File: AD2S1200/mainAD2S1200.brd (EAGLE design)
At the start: 100 x 80 mm, 36 parts, among them IC1 OPA1013D, IC2 OPA1013D, Q1(9235.11QRTZ) 8.192, X1 22-23-2041

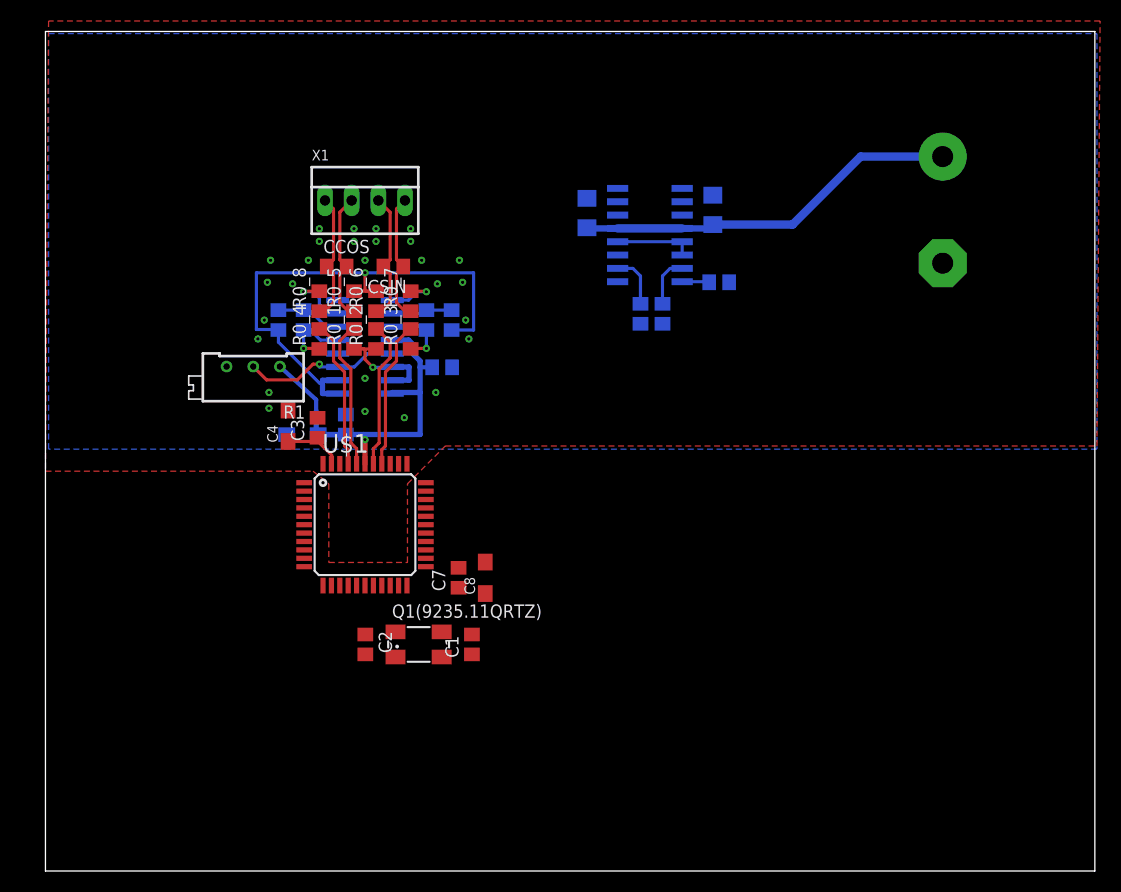
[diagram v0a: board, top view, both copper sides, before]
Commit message: Ok
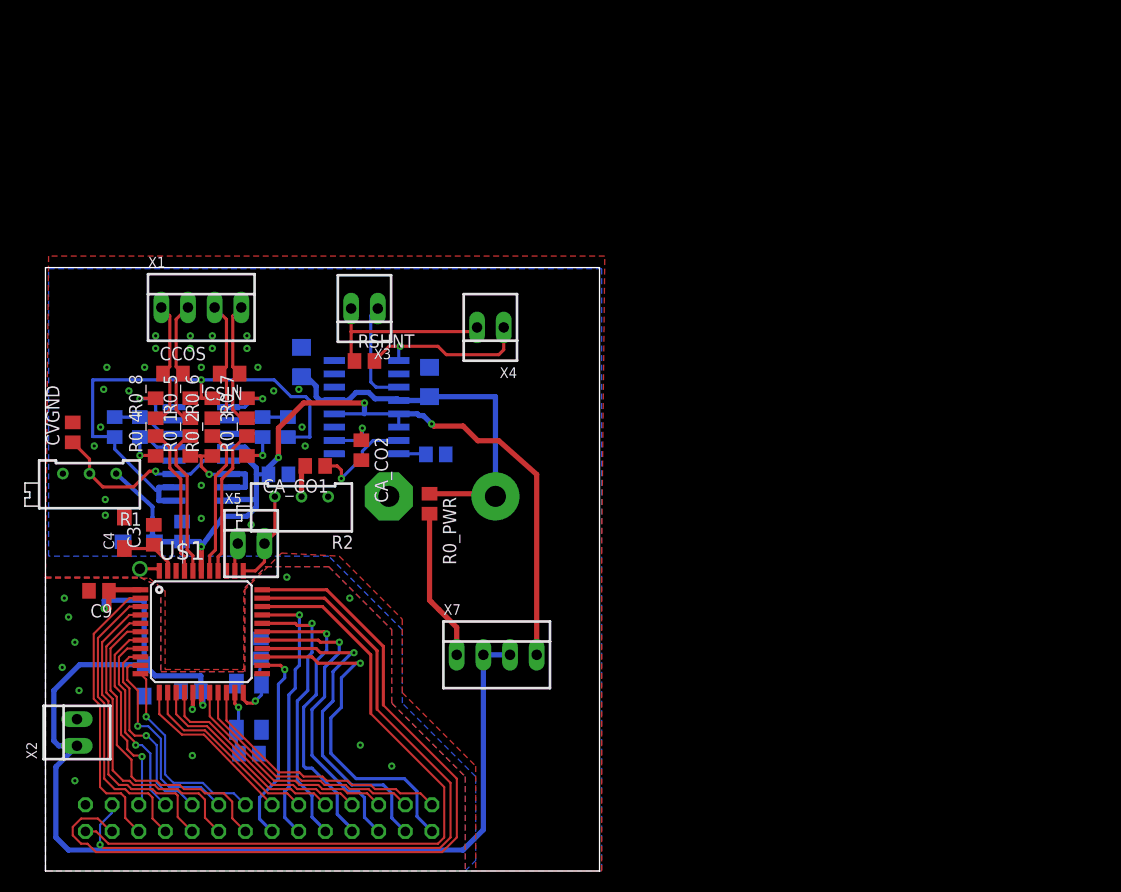
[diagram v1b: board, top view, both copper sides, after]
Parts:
- added C9: 100n, rcl:C0805
- added CVGND: (no value), rcl:C0805
- added R0_PWR, RSHNT: (no value), resistor:R0805
- added R2: (no value), resistor:RTRIM64X
- added SV3, SV4: (no value), con-ml:ML14
- added X2, X3, X4, X5: 22-23-2021, con-molex:22-23-2021
- added X7: 22-23-2041, con-molex:22-23-2041
- moved CA1 55.0 mm to (37.8, 35.7), turned to 0 degrees
- moved CA_CO1 36.1 mm to (25.7, 38.6), flipped to the top, turned to 180 degrees
- moved C8 33.9 mm to (9.41, 18.2), flipped to the bottom, turned to 270 degrees
- moved CA3 31.6 mm to (36.6, 46.6)
- moved CA4 31.6 mm to (37.2, 39.7)
- moved PAM1 31.6 mm to (30.6, 44.2)
- moved CA2 30.7 mm to (24.4, 48.5)
- moved CA_CO2 29.6 mm to (30.1, 40.1), flipped to the top
- moved C7 27.7 mm to (13.9, 17.1), flipped to the bottom, turned to 0 degrees
- moved C1 20.1 mm to (20.5, 21.2), flipped to the bottom, turned to 270 degrees
- moved C3 18.6 mm to (10.3, 32.0)
- moved C4 18.6 mm to (7.52, 32.2)
- moved C5 18.6 mm to (13.0, 32.3)
- moved R0_4 18.6 mm to (10.5, 40.5)
- moved RG_COS_1 18.6 mm to (9.00, 42.3)
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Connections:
- new net N$15: SV4.2, U$1.20
- new net N$18: SV4.4, U$1.19
- new net N$21: SV4.6, U$1.18
- new net N$22: SV4.12, U$1.13
- new net N$23: SV4.14, U$1.12
- new net N$24: SV4.8, U$1.15
- new net N$25: SV4.10, U$1.14
- new net N$26: SV3.5, U$1.7
- new net N$27: SV3.7, U$1.8
- new net N$28: SV3.9, U$1.9
- new net N$29: SV3.11, U$1.10
- new net N$30: SV3.13, U$1.11
- new net N$31: SV4.11, U$1.30
- new net N$32: SV4.7, U$1.28
- new net N$33: SV4.9, U$1.29
- new net N$34: SV4.5, U$1.27
- new net N$35: SV4.3, U$1.26
- new net N$36: SV4.1, U$1.25
- new net N$37: SV4.13, U$1.24
- new net N$38: SV3.6, U$1.2
- new net N$39: SV3.8, U$1.3
- new net N$40: SV3.10, U$1.4
- new net N$41: SV3.12, U$1.5
- new net N$42: SV3.14, U$1.6
- new net N$43: SV3.4, U$1.33
- new net N$44: SV3.2, U$1.31
- new net N$45: SV3.3, U$1.32
- new net N$46: CA_CO1.2, R2.2
- new net N$47: RSHNT.1, X3.2, X4.2
- new net N$48: CA1.+, CA2.1, CA3.1, PAM1.13, PAM1.4, R0_PWR.1
- new net N$49: R0_PWR.2, X7.1
- new net N$50: U$1.44
- net !EXC: now also X5.1; no longer CA_CO2.2
- net +5V: now also C9.1, X2.1, X7.2, X7.3; no longer CA1.+, CA2.1, CA3.1, PAM1.13, PAM1.4
- net EXC: now also R2.3, X5.2; no longer CA_CO1.2
- net GND: now also C9.2, SV3.1, X2.2
- net GNDA: now also CA_CO2.2, CVGND.2, R2.1
- net N$14: now also CVGND.1
- net N$8: now also RSHNT.2, X4.1
- net N$9: now also X3.1
- net VDD: now also X7.4
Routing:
- net N$43: track 0.00 -> 78.1 mm
- net +5V: track 36.8 -> 113.7 mm, vias 0 -> 2
- net N$45: track 0.00 -> 72.0 mm, vias 0 -> 1
- net N$44: track 0.00 -> 67.5 mm
- net VDD: track 45.7 -> 91.7 mm, vias 1 -> 4
- net N$48: track 0.00 -> 36.7 mm
- net N$36: track 0.00 -> 33.7 mm, vias 0 -> 1
- net N$35: track 0.00 -> 32.3 mm, vias 0 -> 1
- net N$42: track 0.00 -> 30.5 mm
- net N$34: track 0.00 -> 29.8 mm, vias 0 -> 1
- net N$41: track 0.00 -> 29.7 mm
- net N$40: track 0.00 -> 29.0 mm
- net N$32: track 0.00 -> 28.2 mm, vias 0 -> 1
- net N$39: track 0.00 -> 28.0 mm
- net N$38: track 0.00 -> 27.3 mm
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- added copper zone on layer 1, net GND
- added copper zone on layer 16, net GND
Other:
- board size 100 x 80 mm -> 52.8 x 57.5 mm
